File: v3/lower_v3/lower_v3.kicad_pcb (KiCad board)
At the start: 2 copper layers, 38.1 x 71.1 mm, 5 parts, among them J1 Conn_01x09_MountingPin, J2 Conn_01x09_MountingPin, J4 Conn_01x02_Male, U1 ESP32-DEVKIT-V1

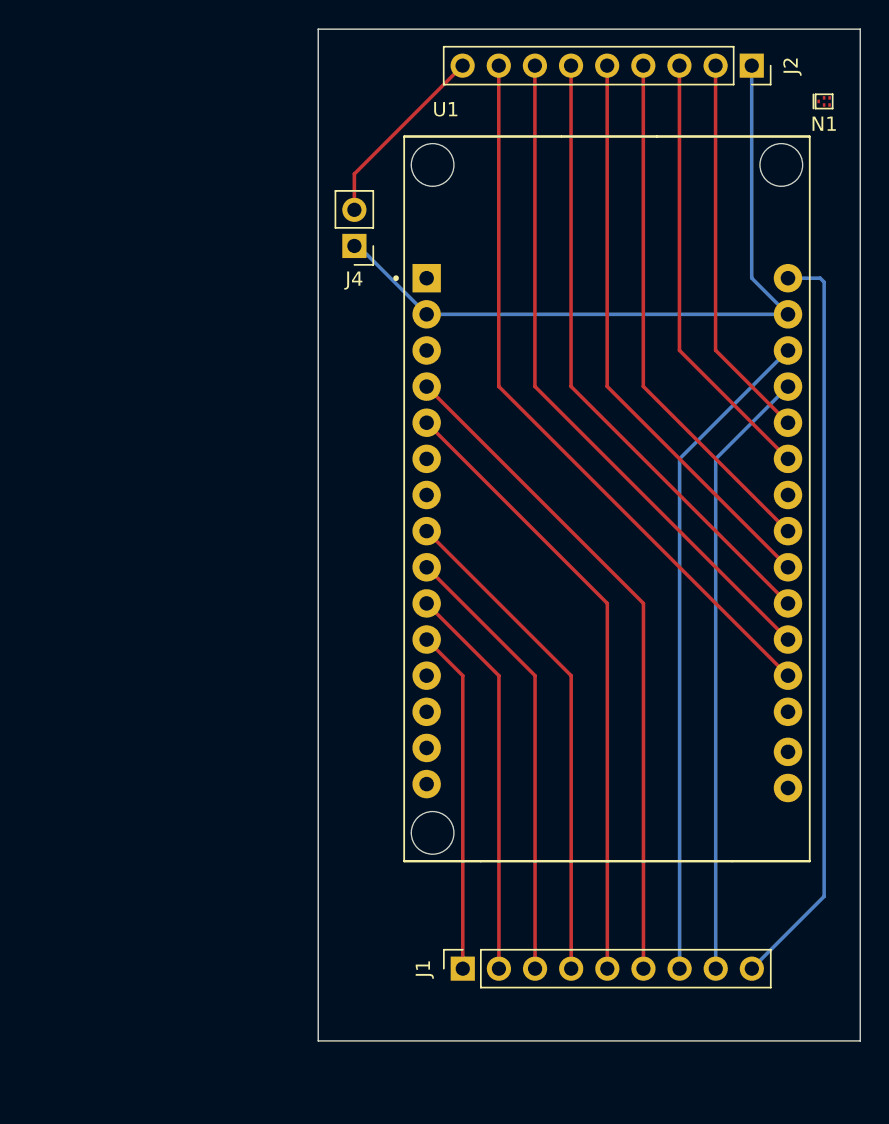
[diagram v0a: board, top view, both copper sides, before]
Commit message: Complete Toast PCB
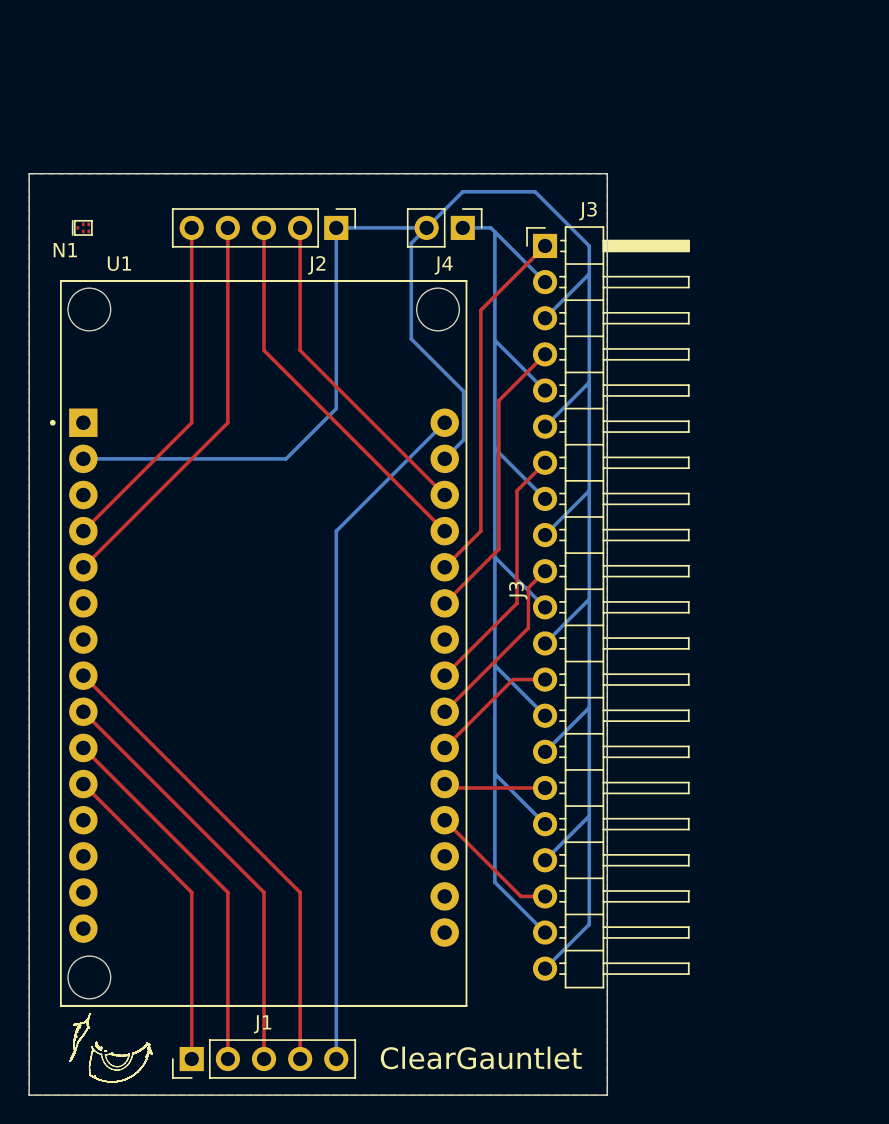
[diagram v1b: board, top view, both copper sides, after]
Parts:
- added J3: Conn_01x21, Connector_PinHeader_2.54mm:PinHeader_1x21_P2.54mm_Horizontal, F.Cu at (150.6, 78.7)
- J1, J2: value Conn_01x09_MountingPin -> Conn_01x05_Male; footprint Connector_PinSocket_2.54mm:PinSocket_1x09_P2.54mm_Vertical -> Connector_PinHeader_2.54mm:PinHeader_1x05_P2.54mm_Vertical
- moved N1 52.8 mm to (118.1, 77.5)
- moved J2 31.4 mm to (135.9, 77.5)
- moved U1 26.2 mm to (130.8, 106.7)
- moved J1 20.1 mm to (125.7, 135.9)
- moved J4 7.73 mm to (144.8, 77.5), turned to -90 degrees
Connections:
- J1 pad 5: Net-(J1-Pad5) -> Net-(U1-Pad30)
- J2 pad 2: Net-(J2-Pad2) -> Net-(U1-Pad28)
- J2 pad 3: Net-(J2-Pad3) -> Net-(U1-Pad27)
- J2 pad 4: Net-(J2-Pad4) -> Net-(U1-Pad5)
- J2 pad 5: Net-(J2-Pad5) -> Net-(U1-Pad4)
- J4 pad 1: GND -> Net-(J4-Pad1)
- J4 pad 2: Net-(J2-Pad9) -> GND
- U1 pad 19: Net-(J2-Pad8) -> Net-(U1-Pad19)
- U1 pad 20: Net-(J2-Pad7) -> Net-(U1-Pad20)
- U1 pad 21: Net-(J2-Pad6) -> Net-(U1-Pad21)
- U1 pad 22: Net-(J2-Pad5) -> Net-(U1-Pad22)
- U1 pad 23: Net-(J2-Pad4) -> Net-(U1-Pad23)
- U1 pad 25: Net-(J2-Pad3) -> Net-(U1-Pad25)
- U1 pad 26: Net-(J2-Pad2) -> Net-(U1-Pad26)
- U1 pad 27: Net-(J1-Pad8) -> Net-(U1-Pad27)
- U1 pad 28: Net-(J1-Pad7) -> Net-(U1-Pad28)
- U1 pad 30: Net-(J1-Pad9) -> Net-(U1-Pad30)
- U1 pad 4: Net-(J1-Pad6) -> Net-(U1-Pad4)
- U1 pad 5: Net-(J1-Pad5) -> Net-(U1-Pad5)
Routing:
- net GND: track 51.0 -> 149.5 mm
- net Net-(J4-Pad1): track 0.00 -> 83.0 mm
- net Net-(J1-Pad9): track 53.0 -> 0.00 mm
- net Net-(J2-Pad8): track 51.3 -> 0.00 mm
- net Net-(U1-Pad30): track 0.00 -> 47.9 mm
- net Net-(J2-Pad7): track 47.7 -> 0.00 mm
- net Net-(J1-Pad6): track 47.2 -> 0.00 mm
- net Net-(J1-Pad7): track 46.6 -> 0.00 mm
- net Net-(J2-Pad6): track 44.1 -> 0.00 mm
- net Net-(J1-Pad5): track 43.6 -> 0.00 mm
- net Net-(J1-Pad8): track 43.0 -> 0.00 mm
- net Net-(J2-Pad5): track 40.5 -> 0.00 mm
- net Net-(J2-Pad4): track 36.9 -> 0.00 mm
- net Net-(J2-Pad3): track 30.8 -> 0.00 mm
- net Net-(U1-Pad5): track 0.00 -> 28.1 mm
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- added copper zone on B.Cu, net GND
- added copper zone on F.Cu, net GND
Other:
- board size 38.1 x 71.1 mm -> 40.6 x 64.8 mm
- board text added: "ClearGauntlet"
